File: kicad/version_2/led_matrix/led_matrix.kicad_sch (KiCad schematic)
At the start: 82 parts, among them Q1 IRF540N, Q2 IRF540N, Q3 IRF540N, Q4 IRF540N, Q5 IRF540N, Q6 IRF540N, Q7 IRF540N, Q9 IRF540N, SW1 SW_DIP_x01

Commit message: Improved readme
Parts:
- removed C1: C, Capacitor_THT:CP_Radial_D4.0mm_P2.00mm, symbol Device:C
- removed D1, D2, D3: LED, LED_THT:LED_D3.0mm, symbol Device:LED
- removed R1, R17, R18, R19, R2, R3, R4: R, custom_footprint_library:0.4_pitch_resistor, symbol Device:R
- removed U1: ~, Connector_PinHeader_2.54mm:PinHeader_1x16_P2.54mm_Vertical, symbol custom_symbol_lib:connector_16_bit
- removed U14, U26: ~, Package_DIP:DIP-28_W15.24mm, symbol custom_symbol_lib:32Kx8_sram
- removed U15: ~, Package_DIP:DIP-14_W7.62mm, symbol custom_symbol_lib:OP_AMP_quad
- removed U16, U3, U32, U43, U44, U51, U52: ~, Package_DIP:DIP-20_W7.62mm, symbol custom_symbol_lib:rising_edge_8_bit_latch
- removed U17, U25: ~, Package_DIP:DIP-16_W7.62mm, symbol custom_symbol_lib:8_bit_counter
- removed U2: ~, Connector_PinHeader_2.54mm:PinHeader_1x03_P2.54mm_Vertical, symbol custom_symbol_lib:power_and_clk
- removed U27, U28: ~, Package_DIP:DIP-16_W7.62mm, symbol custom_symbol_lib:multiplexer_8_bit
- removed U29: ~, Package_DIP:DIP-14_W7.62mm, symbol custom_symbol_lib:quad_OR
- removed U30, U46: ~, Package_DIP:DIP-14_W7.62mm, symbol custom_symbol_lib:6xNOT
- removed U31: ~, Package_DIP:DIP-20_W7.62mm, symbol custom_symbol_lib:8_bit_transparent_latch
- removed U34, U35, U36, U37, U38, U39, U40, U41, U42: ~, custom_footprint_library:jumper, symbol custom_symbol_lib:jumper
- removed U45, U47, U54: ~, Package_DIP:DIP-14_W7.62mm, symbol custom_symbol_lib:quad_and
- removed U48, U53: ~, Package_DIP:DIP-14_W7.62mm, symbol custom_symbol_lib:dual_4_input_OR
- removed U49: ~, Package_DIP:DIP-14_W7.62mm, symbol custom_symbol_lib:dual_latch
- added U1: ~, Connector_PinHeader_2.54mm:PinHeader_1x13_P2.54mm_Vertical, symbol custom_symbol_lib:led_matrix_connector
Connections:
- net at Q1.2 (D), Q2.2 (D), Q3.2 (D)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: now also U1.1 (V+), U1.2 (V+)
- net at R10.2, R11.2, R12.2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: now also U1.12 (GND), U1.13 (GND)
- net at U10.2 (D_in), U12.2 (D_in), U13.2 (D_in)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: now also U1.3 (Data)
- net at U10.3 (CLK), U12.3 (CLK), U13.3 (CLK)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: now also U1.4 (CLK)
- net at U24.1 (A0): now also U1.6 (Driver_A0)
- net at U24.2 (A1): now also U1.7 (Driver_A1)
- net at U24.3 (A2): now also U1.8 (Driver_A2)
- net at U24.6 (E1): now also U1.5 (Driver_LE)
- net at U33.1 (A0): now also U1.9 (Row_A0)
- net at U33.2 (A1): now also U1.10 (Row_A1)
- net at U33.3 (A2): now also U1.11 (Row_A2)
- no-connect marks 35 -> 8
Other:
- note removed: "<- Mem write"
- note removed: "Address"
- note removed: "C-Clk En# (partial) & D-Clk En#"
- note removed: "CLK"
- note removed: "CLK#"
- note removed: "Control latch CLK"
- note removed: "Counter enable"
- note removed: "Data even columns"
- note removed: "Data odd columns"
- note removed: "High byte OE for mem write"
- note removed: "Low byte OE for mem write"
- note removed: "Mem read"
- note removed: "Mem write - Set data"
- note removed: "The entire 16-bit word needs to be reversed when shifted into the shift register. Which is why each byte is individually reversed, then the MSB of the bit address is used backwards when enabling each multiplexer."

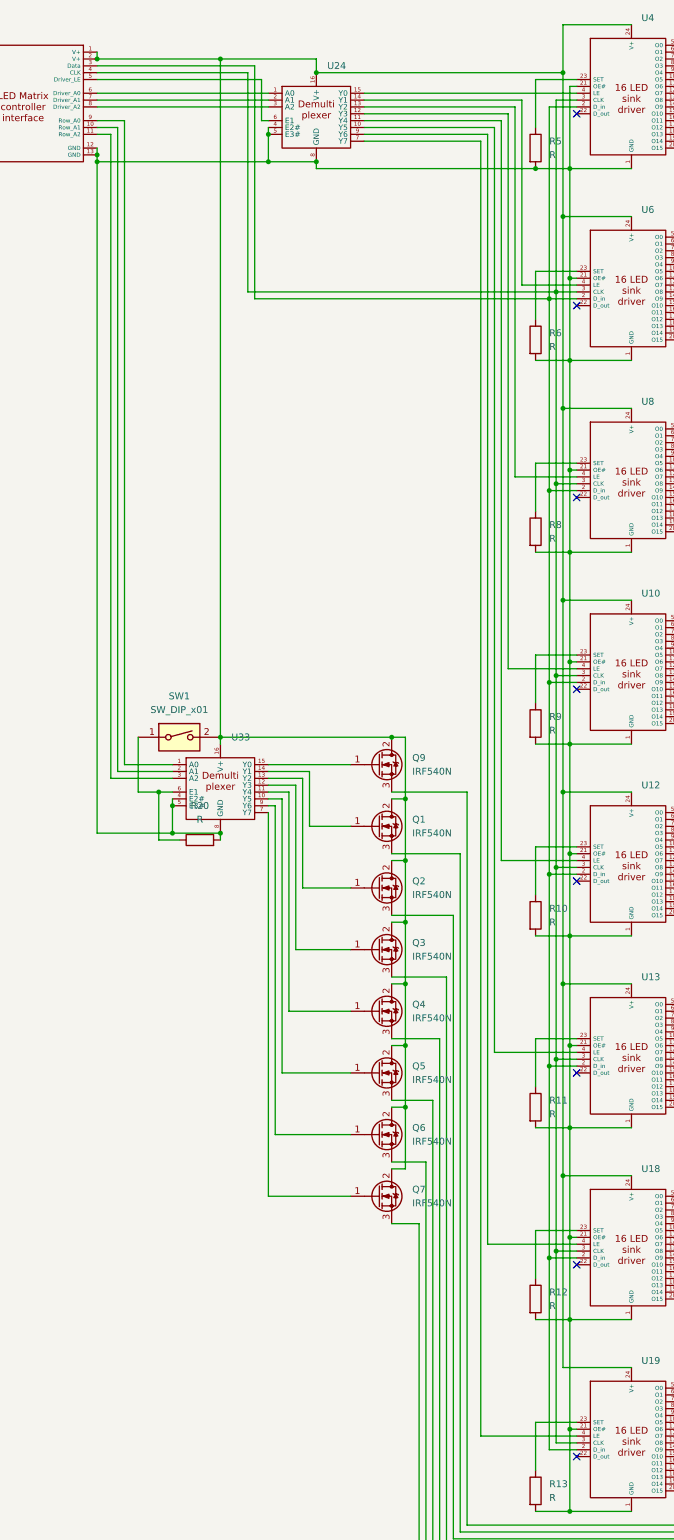
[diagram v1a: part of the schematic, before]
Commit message: Fixed led matrix board
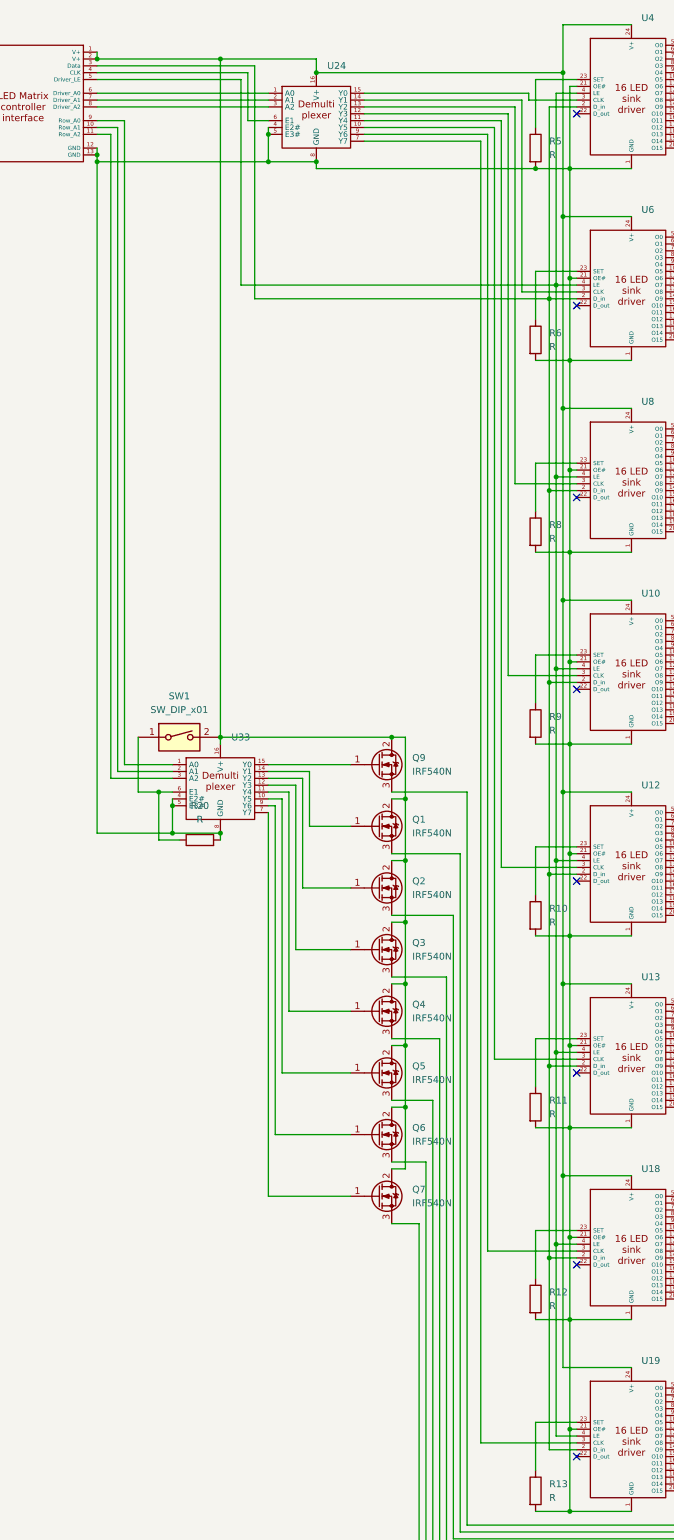
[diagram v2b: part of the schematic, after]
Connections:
- net at U24.10 (Y5): now also U13.3 (CLK); no longer U13.4 (LE)
- net at U12.4 (LE): now also U1.5 (Driver_LE), U10.4 (LE), U13.4 (LE), U18.4 (LE), U19.4 (LE), U4.4 (LE), U6.4 (LE), U8.4 (LE); no longer U24.11 (Y4)
- net at U24.12 (Y3): now also U10.3 (CLK); no longer U10.4 (LE)
- net at U24.13 (Y2): now also U8.3 (CLK); no longer U8.4 (LE)
- net at U24.14 (Y1): now also U6.3 (CLK); no longer U6.4 (LE)
- net at U24.15 (Y0): now also U4.3 (CLK); no longer U4.4 (LE)
- net at U24.6 (E1): now also U1.4 (CLK); no longer U1.5 (Driver_LE)
- net at U24.7 (Y7): now also U19.3 (CLK); no longer U19.4 (LE)
- net at U24.9 (Y6): now also U18.3 (CLK); no longer U18.4 (LE)
- new net: U12.3 (CLK), U24.11 (Y4)
